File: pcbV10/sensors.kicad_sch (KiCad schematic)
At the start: 30 parts, among them J16 BME280, J17 CCS811, J21 QWIIC, U12 BME680, U13 BME280, U15 CCS811, U19 DS18B20, U20 BH1750, U22 AM612, U23 MPU-6050, U3 ICS-43432, U7 DS18B20, U8 HDC1080, X2 XGZP6897D

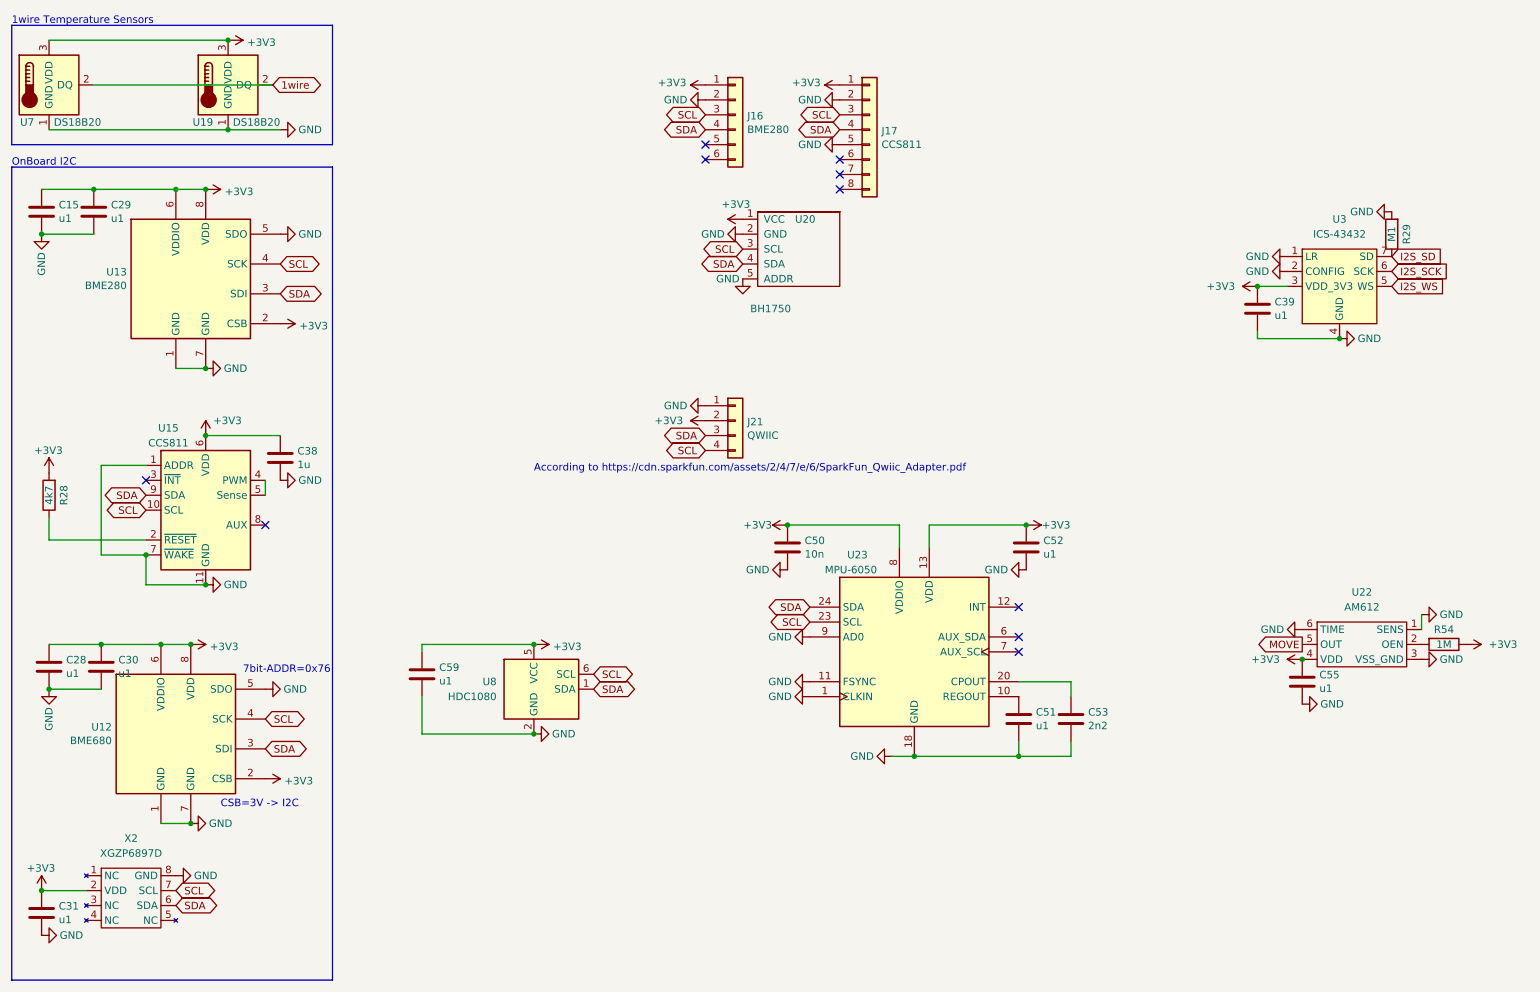
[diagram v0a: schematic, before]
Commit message: Various
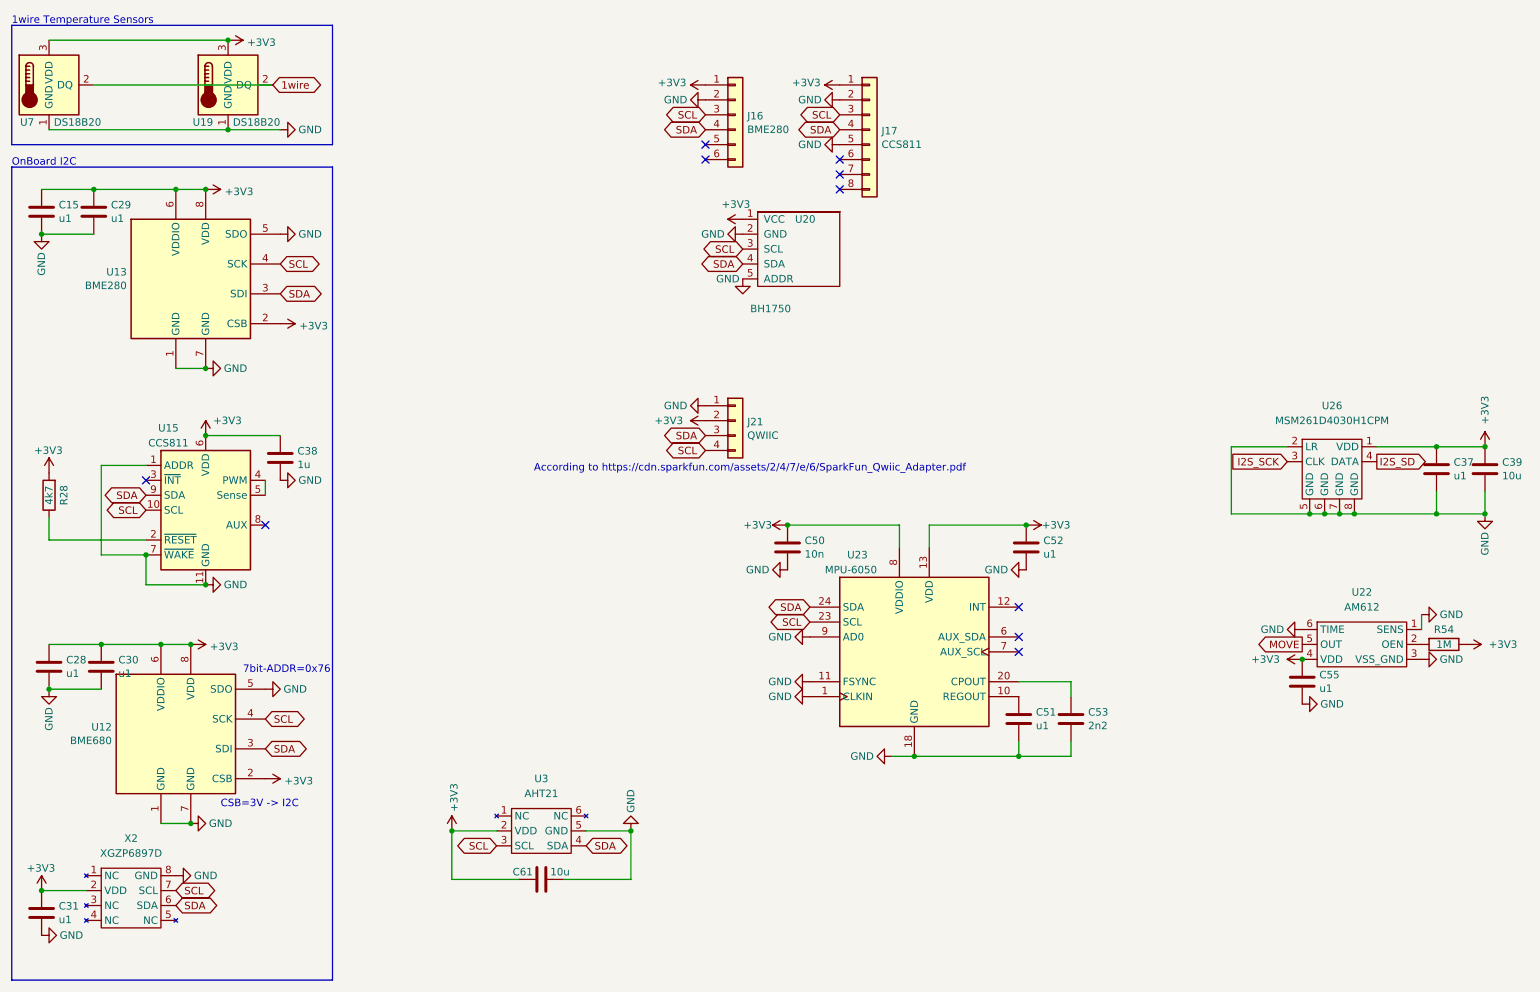
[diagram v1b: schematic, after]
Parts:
- removed C59: u1, Capacitor_SMD:C_0603_1608Metric, symbol Device:C
- removed R29: M1, Resistor_SMD:R_0603_1608Metric, symbol Device:R
- removed U3: ICS-43432, liebler_SEMICONDUCTORS:MIC_ICS-43432, symbol liebler_SEMICONDUCTORS:ICS-43432
- removed U8: HDC1080, Package_SON:Texas_PWSON-N6, symbol Sensor_Humidity:HDC1080
- added C37: u1, Capacitor_SMD:C_0603_1608Metric, symbol Device:C
- added C61: 10u, Capacitor_SMD:C_0603_1608Metric, symbol Device:C
- added U26: MSM261D4030H1CPM, liebler_SEMICONDUCTORS:MSM261D4030H1CPM, symbol liebler_SEMICONDUCTORS:MSM261D4030H1CPM
- added U3: AHT21, liebler_SEMICONDUCTORS:AHT21, symbol liebler_SEMICONDUCTORS:AHT21
- C39: value u1 -> 10u
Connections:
- net +3V3: now also C37.2, C61.1, U26.1 (VDD), U3.2 (VDD)
- net GND: now also C37.1, C61.2, U26.2 (LR), U26.5 (GND), U26.6 (GND), U26.7 (GND), U26.8 (GND), U3.5 (GND)
- net I2S_SCK: now also U26.3 (CLK)
- net I2S_SD: now also U26.4 (DATA)
- net SCL: now also U3.3 (SCL)
- net SDA: now also U3.4 (SDA)
